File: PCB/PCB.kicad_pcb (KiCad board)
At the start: 2 copper layers, 51 x 37.5 mm, 76 parts, among them J1 AudioJack3, J10 Conn_01x01_Pin, J11 Conn_01x01_Pin, J12 Conn_01x01_Pin, J2 USB4105-GF-A, J3 Conn_01x03_Pin, J4 Conn_01x03_Pin, J5 Conn_01x03_Pin, J6 Conn_01x03_Pin, J7 Conn_01x03_Pin, J8 Conn_01x03_Pin, J9 Conn_01x01_Pin, U1 ADP151AUJZ-3.3-R7, U2 MAX41400ATB+T, U3 AD8534ARZ, U6 AD8534ARZ

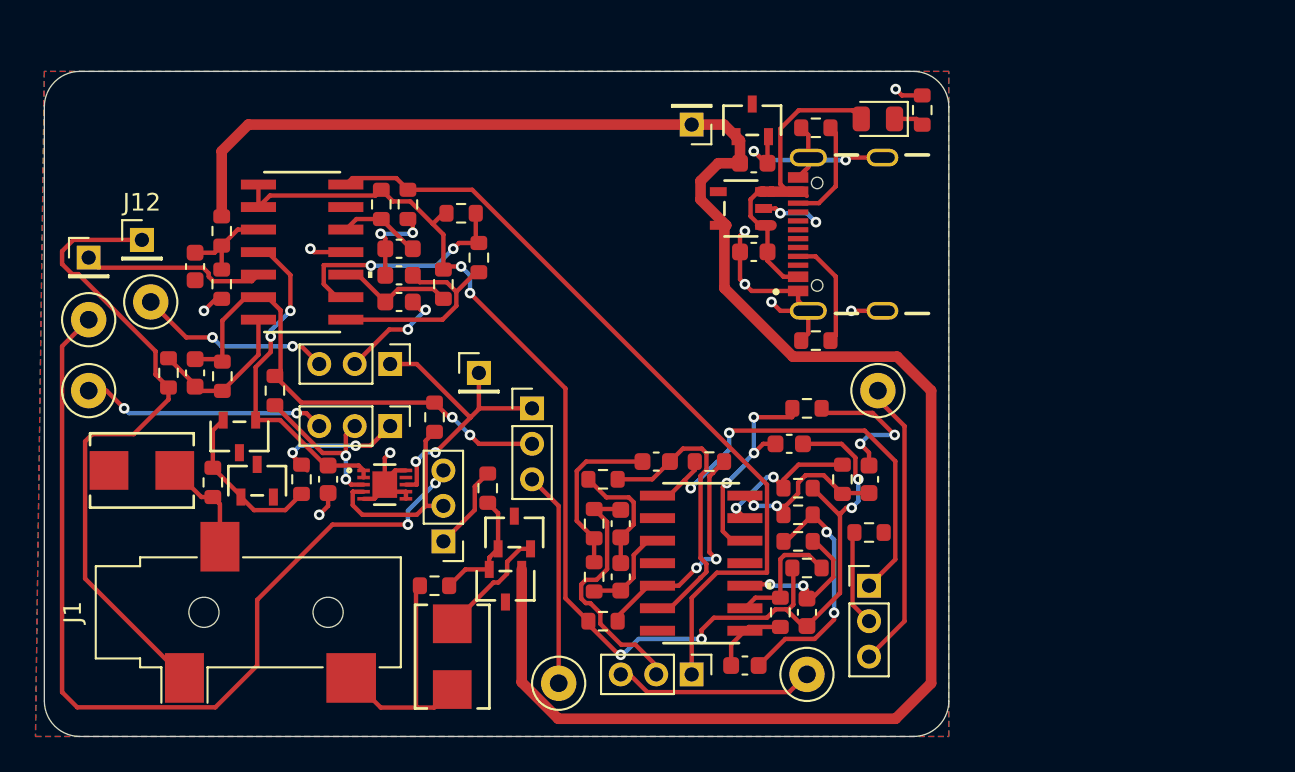
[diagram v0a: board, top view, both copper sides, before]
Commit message: Modificat pcb
Signed-off-by: Andrei Bota <botaandrei69@yahoo.com>
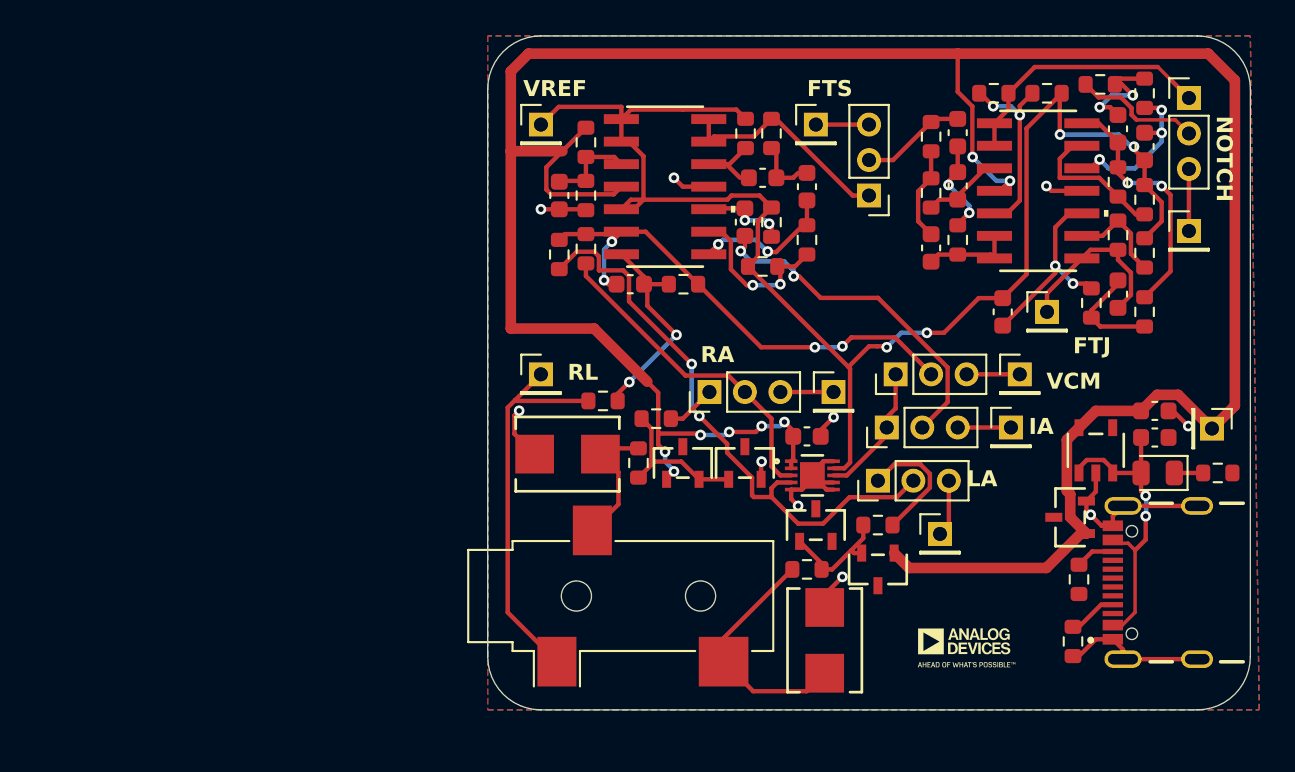
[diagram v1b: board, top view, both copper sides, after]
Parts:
- removed J9: Conn_01x01_Pin, Connector_PinHeader_2.00mm:PinHeader_1x01_P2.00mm_Vertical
- removed TP1, TP2, TP3, TP4, TP5, TP6: TestPoint, TestPoint:TestPoint_Loop_D2.50mm_Drill1.0mm_LowProfile
- added G***: LOGO, ADlogo:adlogo, F.Cu at (155.0, 148.5)
- added J13: Conn_01x01_Pin, Connector_PinHeader_2.00mm:PinHeader_1x01_P2.00mm_Vertical, F.Cu at (153.5, 142.1)
- added J14: Conn_01x01_Pin, Connector_PinHeader_2.00mm:PinHeader_1x01_P2.00mm_Vertical, F.Cu at (147.5, 134.1)
- added J15: Conn_01x01_Pin, Connector_PinHeader_2.00mm:PinHeader_1x01_P2.00mm_Vertical, F.Cu at (158.0, 133.1)
- added J16: Conn_01x01_Pin, Connector_PinHeader_2.00mm:PinHeader_1x01_P2.00mm_Vertical, F.Cu at (157.5, 136.1)
- added J17: Conn_01x01_Pin, Connector_PinHeader_2.00mm:PinHeader_1x01_P2.00mm_Vertical, F.Cu at (146.5, 119.0)
- added J18: Conn_01x01_Pin, Connector_PinHeader_2.00mm:PinHeader_1x01_P2.00mm_Vertical, F.Cu at (167.5, 125.0)
- added J19: Conn_01x01_Pin, Connector_PinHeader_2.00mm:PinHeader_1x01_P2.00mm_Vertical, F.Cu at (159.5, 129.6)
- moved R20 38.9 mm to (159.5, 117.2), turned to 0 degrees
- moved J11 34.0 mm to (168.8, 136.1), turned to -90 degrees
- moved J8 32.9 mm to (167.5, 117.5)
- moved C15 29.7 mm to (163.5, 128.6), turned to 90 degrees
- moved R29 29.5 mm to (161.3, 144.6), turned to 90 degrees
- moved C10 29.1 mm to (154.5, 122.5)
- moved C6 29.1 mm to (154.5, 119.5)
- moved R16 28.9 mm to (153.0, 119.7)
- moved R17 28.8 mm to (153.0, 122.9)
- moved J3 28.8 mm to (149.5, 123.0), turned to 180 degrees
- moved D1 28.7 mm to (160.8, 141.1), turned to 90 degrees
- moved R27 28.5 mm to (163.5, 125.2)
- moved R21 28.4 mm to (162.5, 116.7)
- moved U6 28.3 mm to (159.0, 122.7)
- moved J4 28.2 mm to (150.5, 136.1), turned to 90 degrees
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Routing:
- net SemnalTestLA: track 51.8 -> 3.21 mm, vias 2 -> 0
- net FTS: track 45.2 -> 12.6 mm
- net Vcc: track 125.3 -> 151.7 mm, vias 2 -> 8
- net INAL_IN: track 11.3 -> 33.1 mm, vias 0 -> 2
- net RL: track 37.2 -> 22.3 mm
- net FTS_IN: track 6.24 -> 19.5 mm
- net SemnalTestFTJ: track 15.9 -> 3.50 mm
- net GND: track 52.5 -> 40.7 mm, vias 13 -> 10
- net Net-(U6--INB): track 16.4 -> 5.10 mm
- net SemnalTestRA: track 13.8 -> 3.00 mm, vias 2 -> 0
- net NOTCH: track 25.5 -> 15.3 mm, vias 2 -> 0
- net OutIna: track 17.5 -> 7.59 mm, vias 2 -> 0
- net SemnalTestRL: track 12.1 -> 3.00 mm
- net INAR_IN: track 9.51 -> 18.5 mm, vias 2 -> 0
- net NOTCH_IN: track 14.7 -> 5.96 mm
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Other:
- board size 51 x 37.5 mm -> 43 x 38 mm
- board text added: "Bota Andrei Rev A 04/2026"
- board text added: "FTJ"
- board text added: "FTS"
- board text added: "IA"
- board text added: "LA"
- board text added: "NOTCH"
- board text added: "RA"
- board text added: "RL"
- board text added: "VCM"
- board text added: "VREF"
